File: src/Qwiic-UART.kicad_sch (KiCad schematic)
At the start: 14 parts, among them J1 QWIIC, J2 QWIIC, J3 FTDI, U1 SC16IS740, X1 ECS-2520MVLC-018-BN-TR

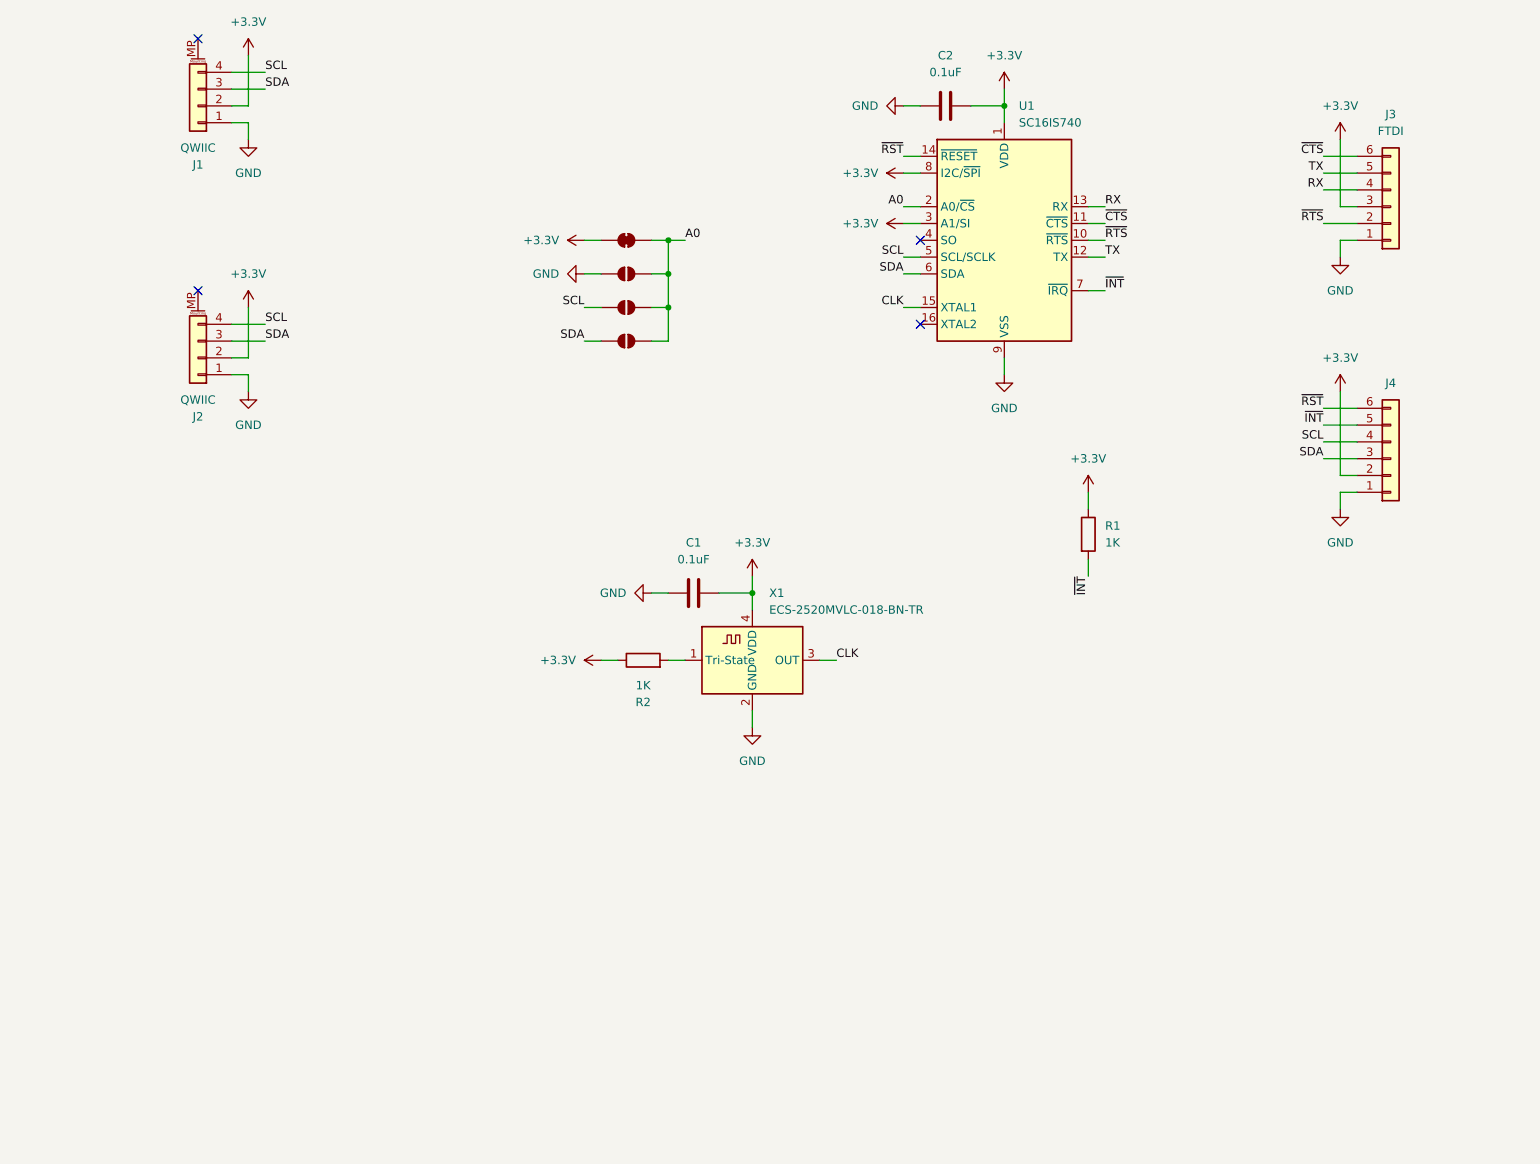
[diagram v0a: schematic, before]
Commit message: Added/generated essential files
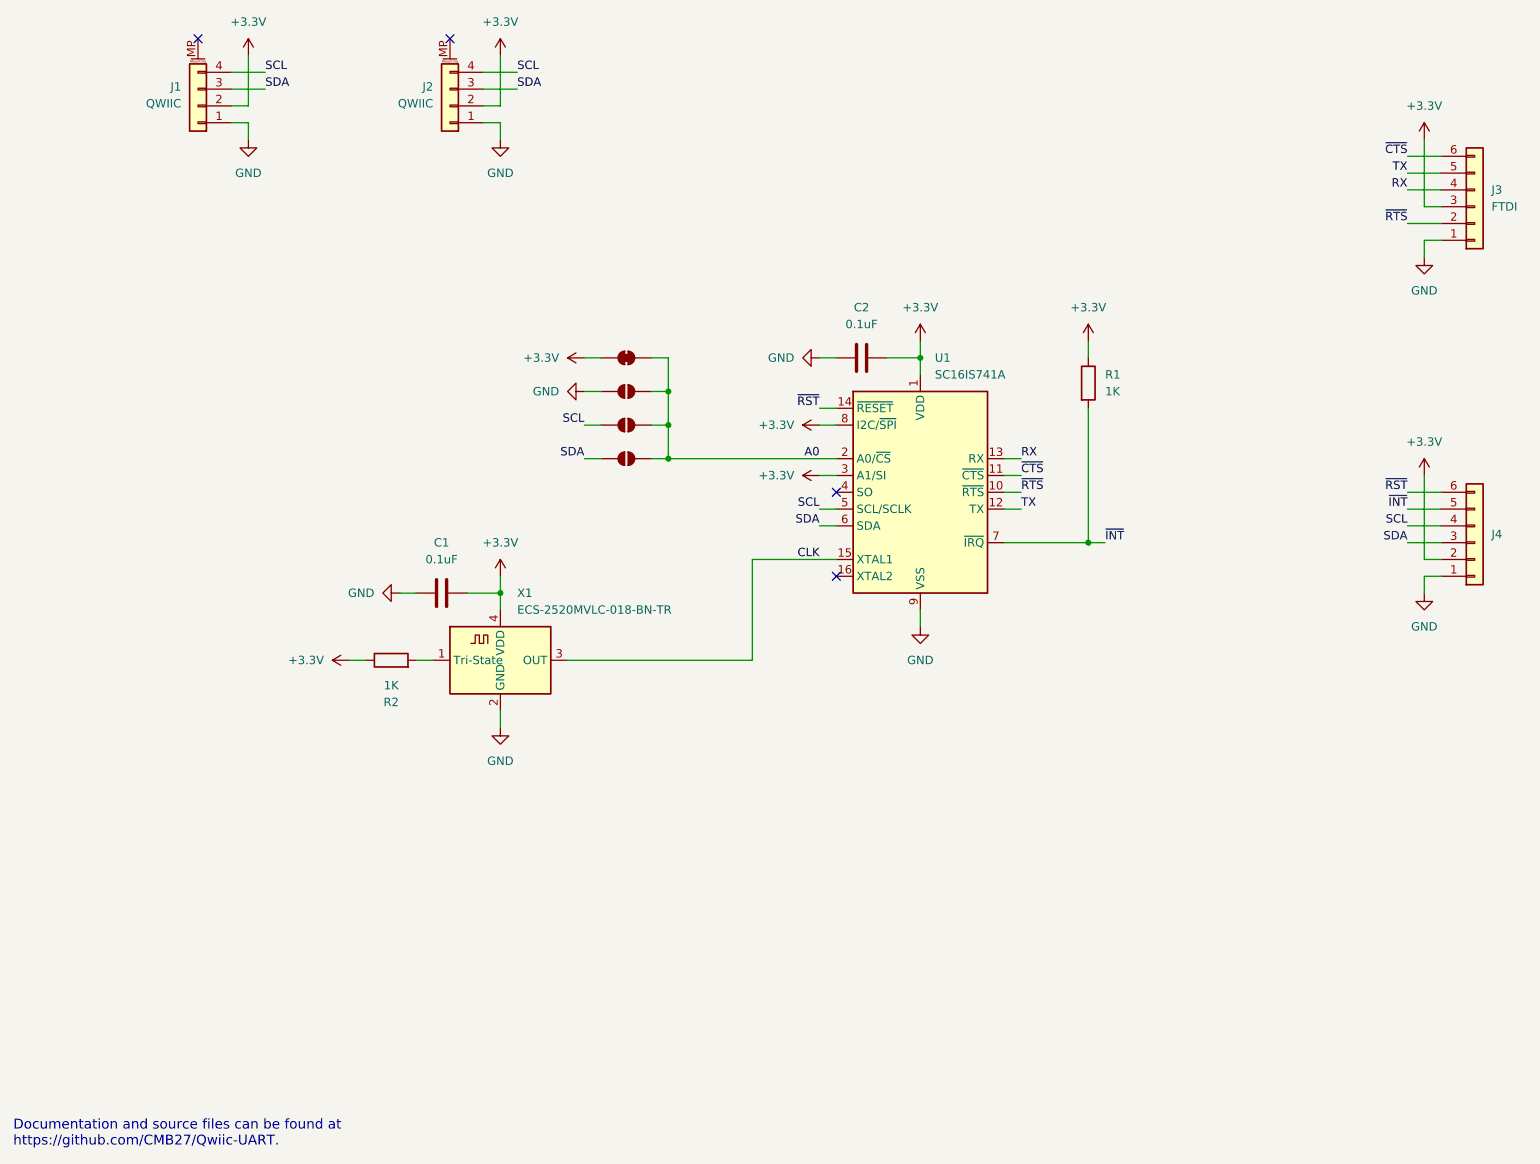
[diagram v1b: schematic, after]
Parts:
- J3, J4: now left out of the parts list
- U1: value SC16IS740 -> SC16IS741A
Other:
- note added: "Documentation and source files can be found at https://github.com/CMB27/Qwiic-UART."
- company: (none) -> Designer: C. M. Bulliner
- title: (none) -> Qwiic UART
- moved on the sheet: C1, C2, J2, J3, J4, R1, R2, U1, X1
